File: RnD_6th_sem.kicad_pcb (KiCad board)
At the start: 2 copper layers, 62.1 x 76.3 mm, 74 parts, among them IC1 2EDF7275KXUMA1, J1 HVDC, J10 MMCX-J-P-H-ST-TH1, J2 PWM, J3 HVDC, J4 Conn_01x06_Female, J5 5V, J6 5V, J7 GND, J8 GND, J9 MMCX-J-P-H-ST-TH1, Q1 IGLD60R190D1, Q2 IGLD60R190D1

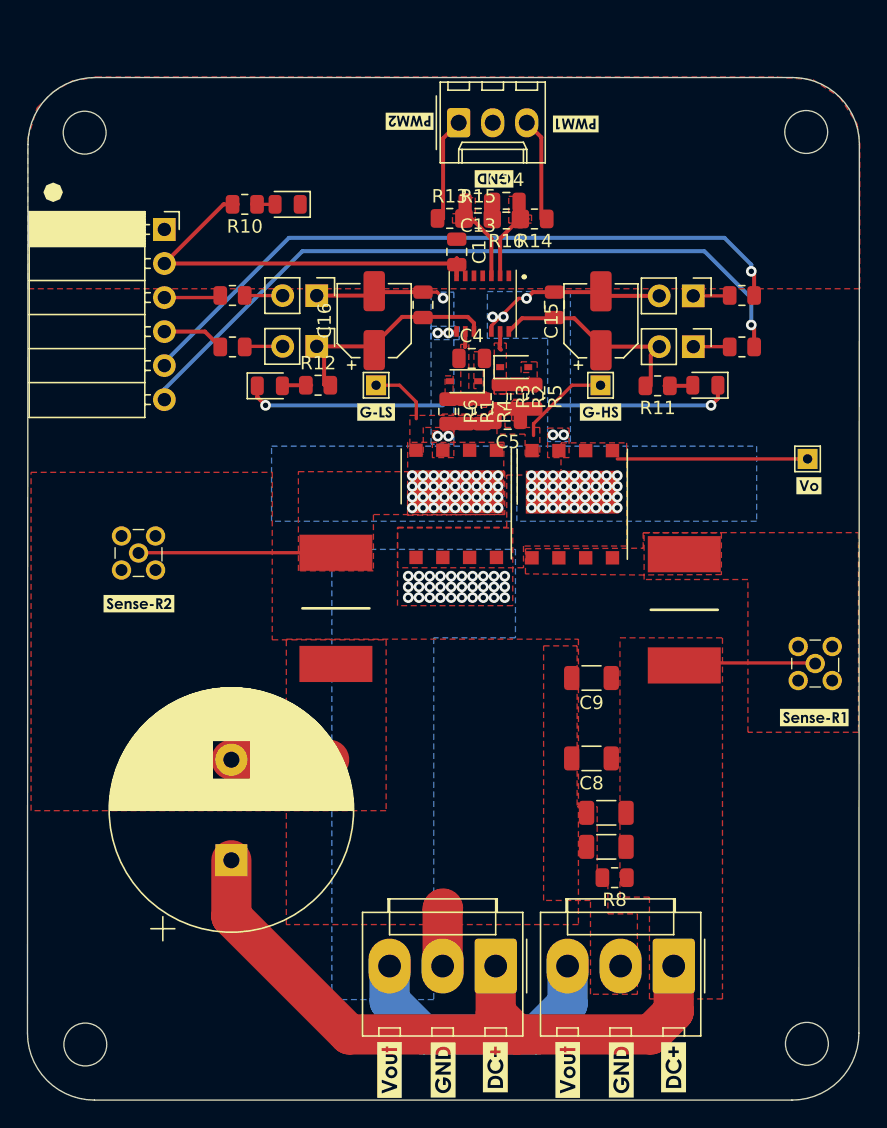
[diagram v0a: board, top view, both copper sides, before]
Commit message: Updated final design
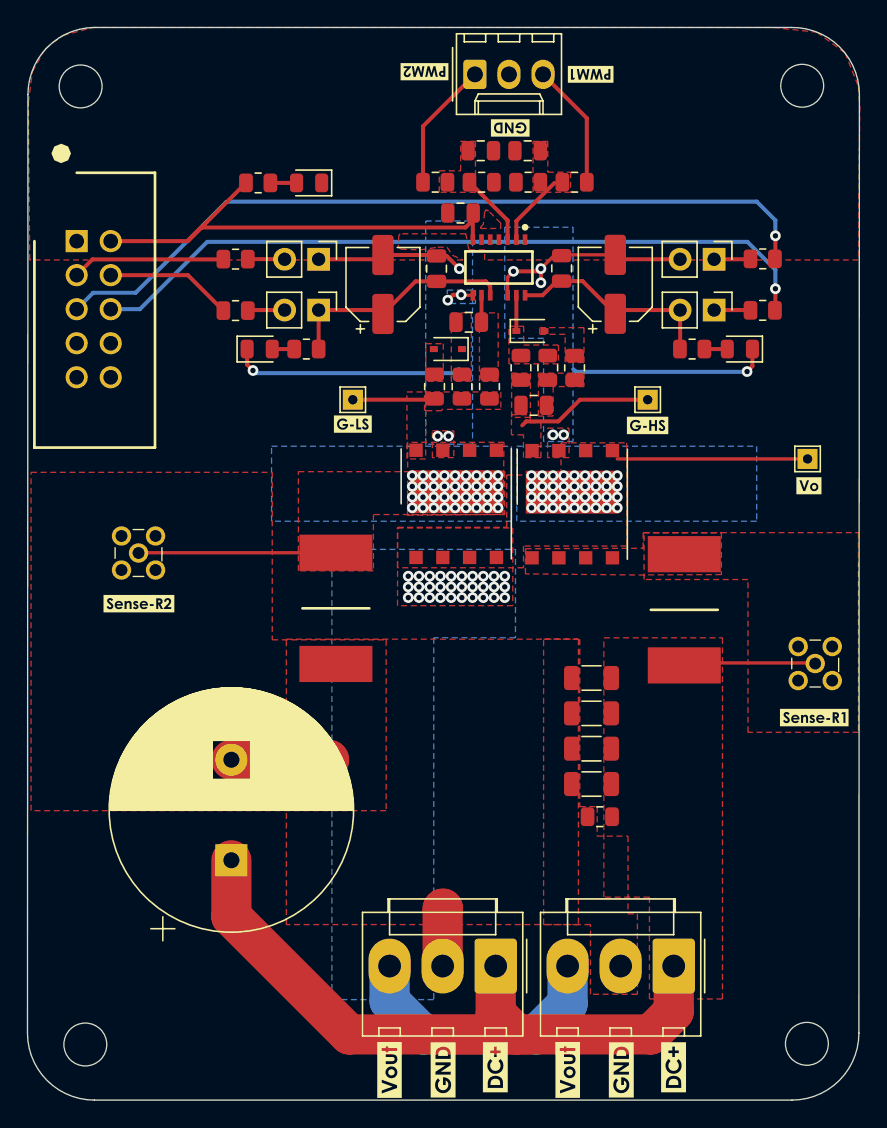
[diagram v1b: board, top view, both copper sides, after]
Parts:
- IC1: footprint 2EDF7275KXUMA1:2EDF7275KXUMA1 -> 2EDF7275K:TFLGA65P500X500X106-14_13N-V
- J4: value Conn_01x06_Female -> Conn_02x05_Odd_Even; footprint Connector_PinSocket_2.54mm:PinSocket_1x06_P2.54mm_Horizontal -> 61201021621:SHDR10W64P254_2X5_2036X885X925P
- moved J4 6.60 mm to (109.4, 61.3), turned to -90 degrees
- moved C6 4.91 mm to (147.9, 99.1)
- moved C7 4.82 mm to (147.9, 101.8)
- moved R8 4.68 mm to (148.5, 104.2)
- moved C14 4.17 mm to (143.1, 54.5)
- moved R14 4.06 mm to (146.6, 56.9)
- moved kibuzzard-63EDD87E 3.99 mm to (141.8, 52.8)
- moved C13 3.92 mm to (139.6, 54.5)
- moved kibuzzard-63EDD841 3.86 mm to (135.4, 48.6)
- moved kibuzzard-63EDD861 3.86 mm to (147.8, 48.8)
- moved J2 3.81 mm to (139.2, 48.8)
- moved R5 3.77 mm to (146.6, 70.7)
- moved R11 3.77 mm to (155.4, 69.3)
- moved D6 3.73 mm to (158.9, 69.3)
- moved TP1 3.68 mm to (152.0, 73.1)
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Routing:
- net Net-(C5-Pad2): track 0.00 -> 10.2 mm
- net Net-(FB1-Pad2): track 51.1 -> 58.9 mm
- net Net-(FB2-Pad1): track 4.23 -> 11.4 mm
- net Net-(C5-Pad1): track 7.07 -> 0.00 mm
- net +3.3V: track 30.6 -> 36.4 mm
- net Net-(FB3-Pad1): track 4.64 -> 9.50 mm
- net gnd-2: track 26.2 -> 30.5 mm
- net gnd-1: track 27.4 -> 31.1 mm
- net Net-(J2-Pad1): track 7.63 -> 9.66 mm
- net Net-(J2-Pad3): track 7.63 -> 9.40 mm
- net Net-(FB4-Pad1): track 54.0 -> 55.6 mm
- net Net-(Q2-Pad8): track 4.77 -> 6.13 mm
- net OUTA: track 1.42 -> 2.66 mm
- net LED2: track 16.6 -> 17.7 mm
- net OUTB: track 1.18 -> 2.02 mm
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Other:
- board size 62.1 x 76.3 mm -> 62.1 x 80 mm
- board text added: "No PWM connector silkscreen review"
- board text removed: "change power loop vias for heat tranfer bottom layer for output right angled connectors for power board 0402 ccomponents connect sense resisots directly to mmcx with test points(research about tt pointys)"
